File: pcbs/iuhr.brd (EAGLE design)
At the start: 38.4 x 23 mm, 73 parts, among them IC1 TPS77033, IC2 MEGA48/88/168-AU, Q1 20.000MHz

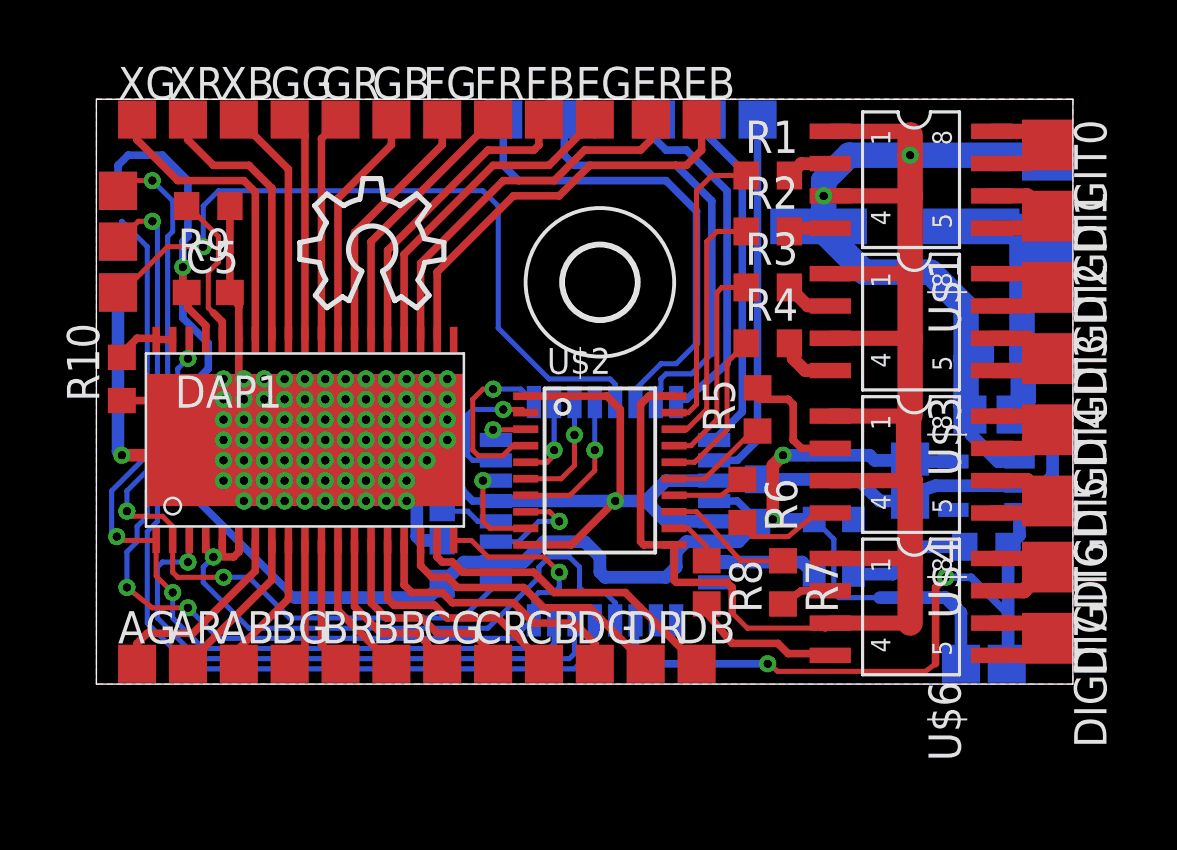
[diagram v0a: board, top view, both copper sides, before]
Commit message: Improved Silkscreen.
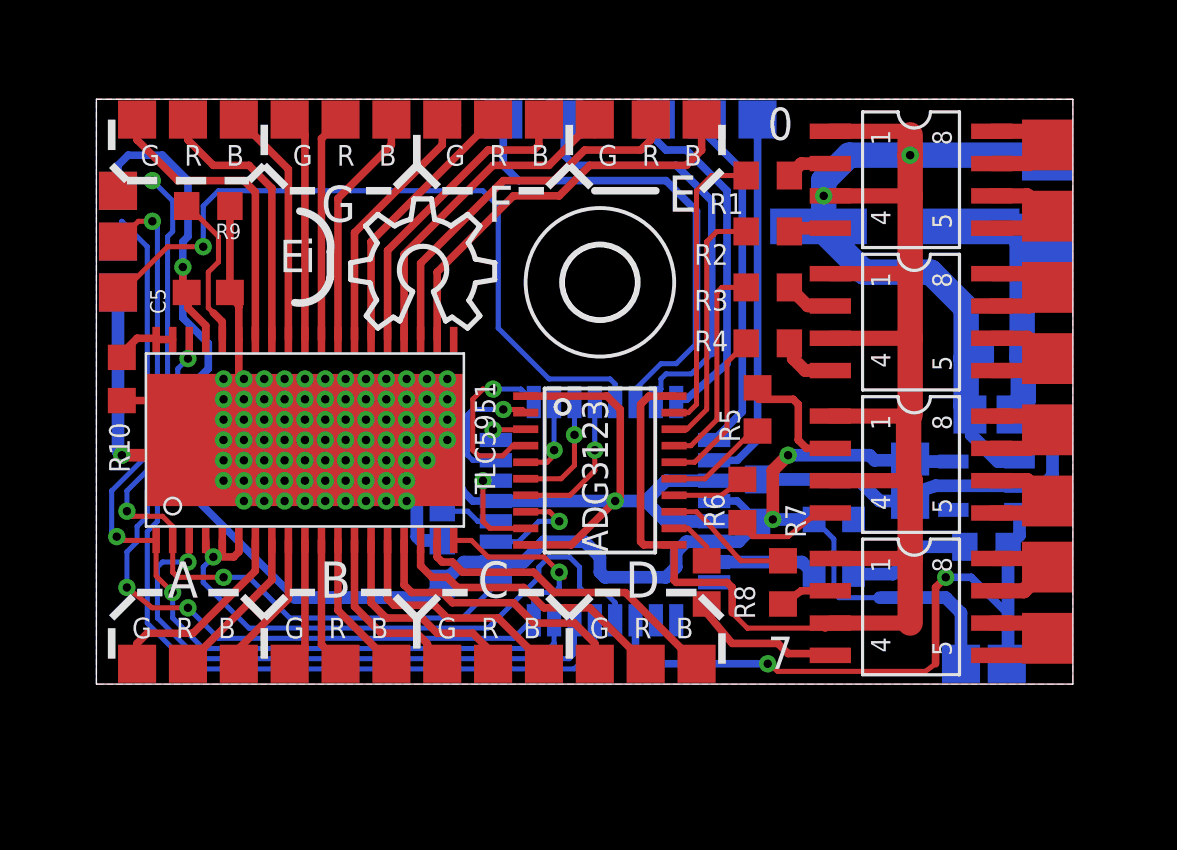
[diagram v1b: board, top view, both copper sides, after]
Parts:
- removed LOGO3: OSHW_LOGO_8MILX0350-NT, ea:OSHW_8X350_NOTEXT
- moved LOGO1 2.15 mm to (10.0, 14.0)
- renumbered DAP1 to TLC5951, IC2 to ATMEGA88PA, U$1 to IRF7104, U$2 to ADG3123
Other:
- board text added: "(C) eKiwi 2013"
- board text added: "+12V"
- board text added: "0"
- board text added: "7"
- board text added: "A"
- board text added: "B"
- board text added: "BTN"
- board text added: "C"
- board text added: "D"
- board text added: "E"
- board text added: "Ei"
- board text added: "Encoder"
- board text added: "F"
- board text added: "G"
- board text added: "G R B"
- board text added: "GND"
- board text added: "ISP"
- board text added: "Licence: CERN OHL v1.2"
- board text added: "ON Button"
- board text added: "UART"
- board text added: "https://github.com/ekiwi/iuhr"
